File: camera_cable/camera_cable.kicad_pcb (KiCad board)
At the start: 4 copper layers, 42.2 x 63.7 mm, 2 parts

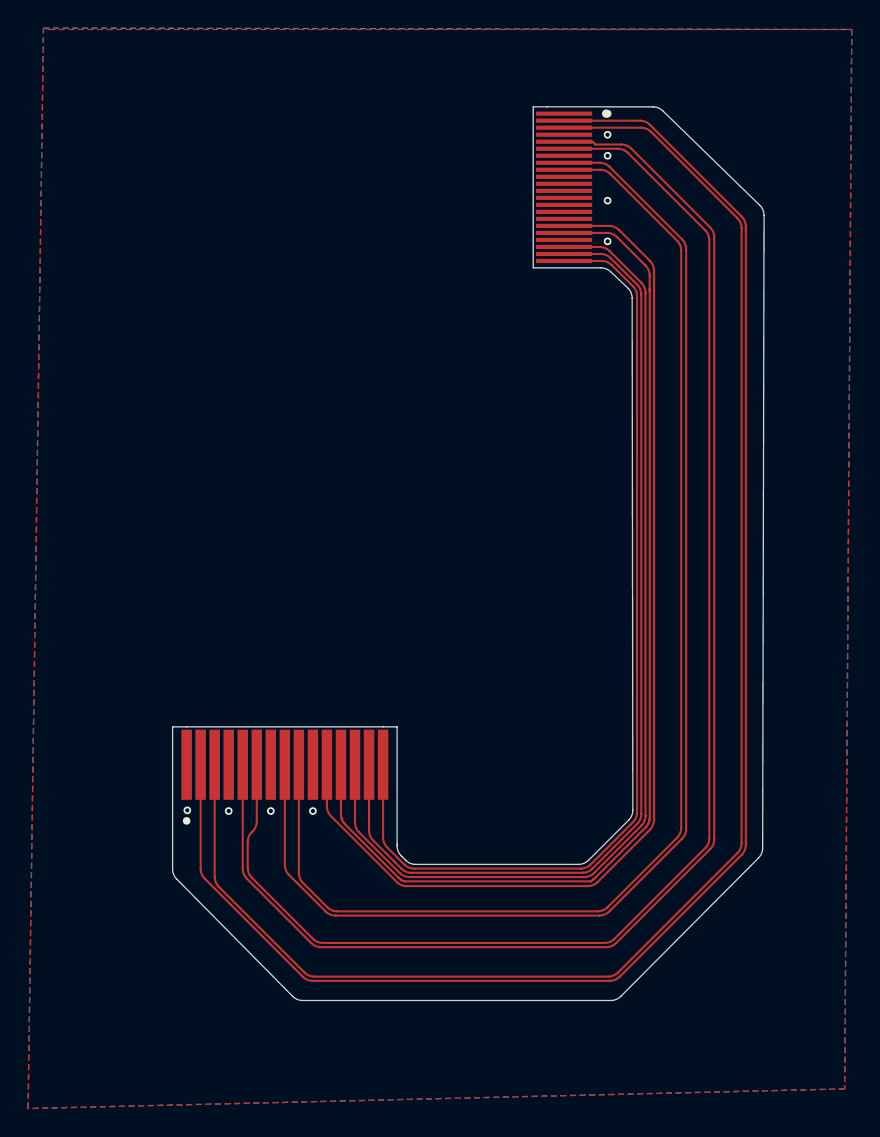
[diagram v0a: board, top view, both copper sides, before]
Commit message: fixed and reordered
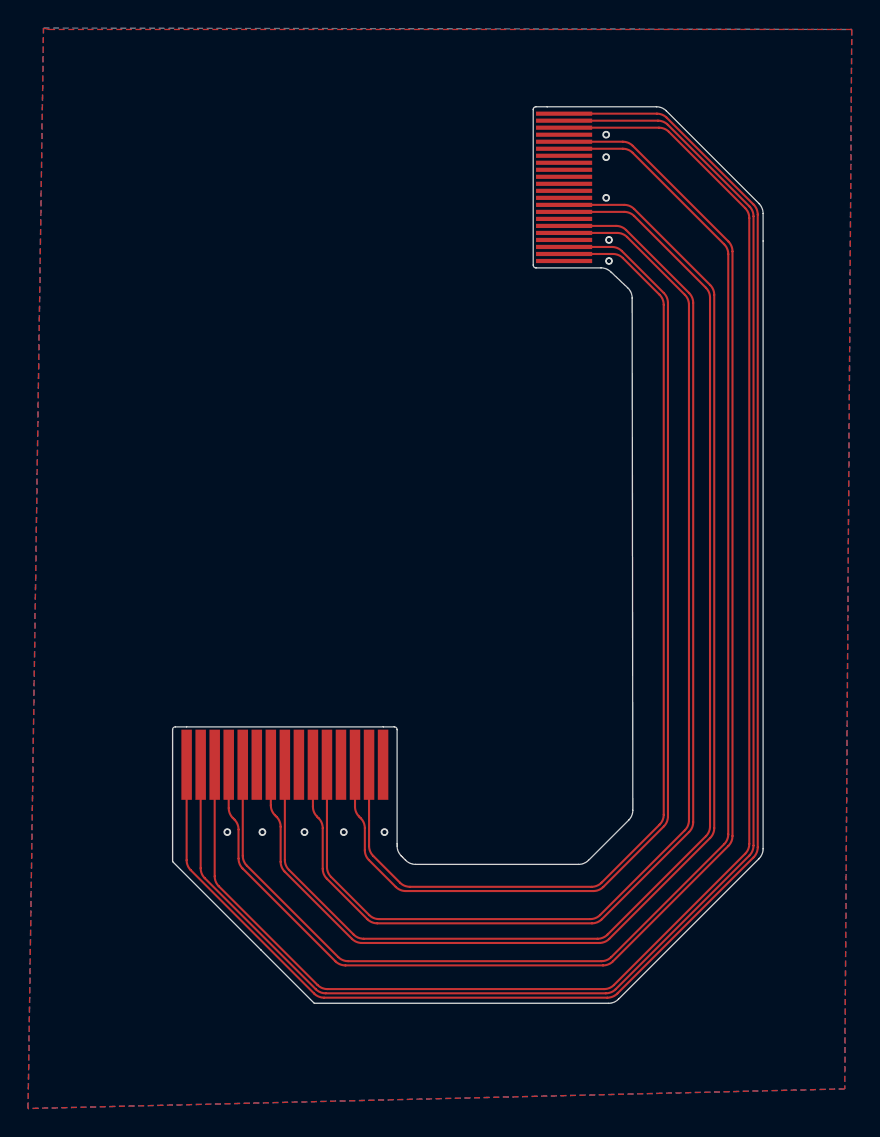
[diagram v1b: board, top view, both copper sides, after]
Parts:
- turned J2 to 90 degrees
- turned j1 to 180 degrees
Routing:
- net Net-(J2-CAM_3v3): track 69.5 -> 118.3 mm
- net Net-(J2-CAM_SDA): track 71.2 -> 116.4 mm
- net Net-(J2-CAM_SCA): track 73.3 -> 114.6 mm
- net Net-(J2-CAM_D0_N): track 114.2 -> 75.5 mm
- net Net-(J2-CAM_D0_P): track 112.3 -> 77.6 mm
- net Net-(J2-CAM_IO1): track 75.9 -> 106.4 mm
- net Net-(J2-CAM_IO0): track 77.9 -> 104.5 mm
- net Net-(J2-CAM_D1_N): track 103.4 -> 85.7 mm
- net Net-(J2-CAM_D1_P): track 101.8 -> 87.5 mm
- net Net-(J2-CAM_CK_P): track 90.9 -> 95.6 mm
- net Net-(J2-CAM_CK_N): track 92.8 -> 93.8 mm
- net GND: track 0.00 -> 0.14 mm, vias 9 -> 10
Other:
- board size 42.2 x 63.7 mm -> 42.1 x 63.9 mm
- board text added: "STIFFENER: 0.2 mm PI"
- board text removed: "STIFFENER: 0.25 mm PI"
